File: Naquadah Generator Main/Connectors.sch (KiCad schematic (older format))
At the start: 23 parts, among them J0 Conn_ISP_Prog, J1 State_Sensing_Conn, J10 Power Board Conn, J2 State_Sensing_Conn

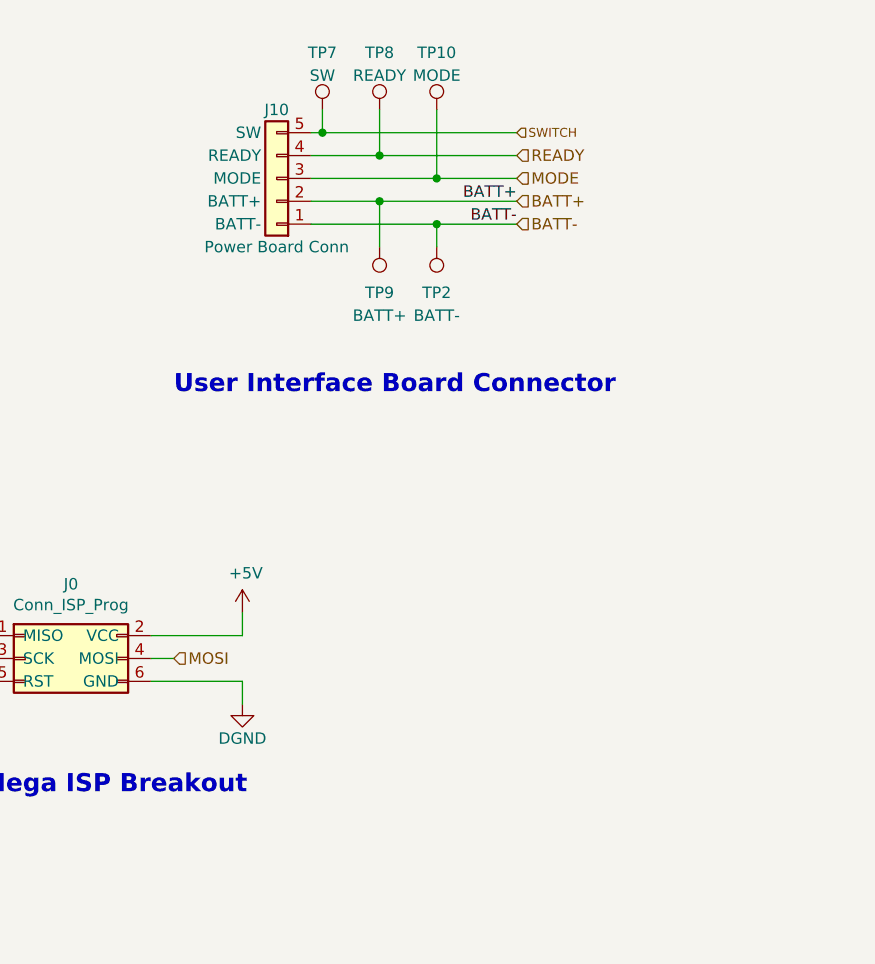
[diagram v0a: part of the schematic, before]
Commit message: Switched to 0603_1608M size for passives
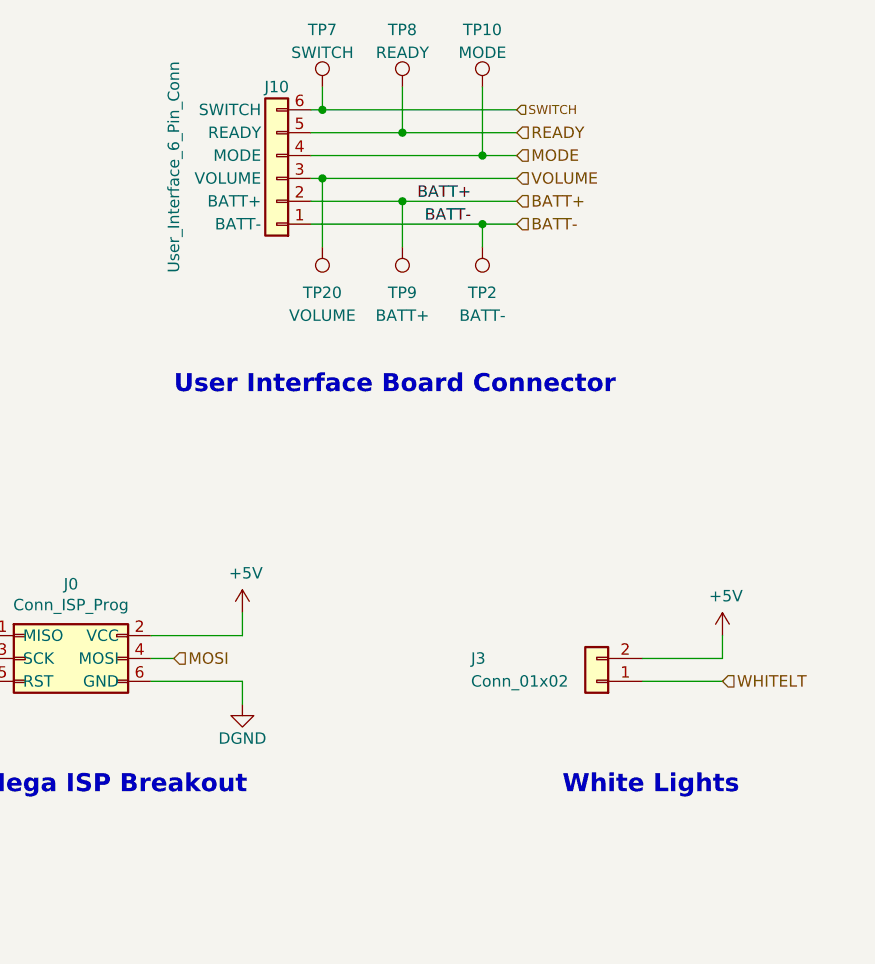
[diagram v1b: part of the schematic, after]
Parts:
- removed J10: Power Board Conn, Naquadah_Generator:Daughter_Board_Vert_5_Pin_JST_Conn, symbol Naquadah_Generator:Power_Daughter_5_Pin_Conn
- added J10: User_Interface_6_Pin_Conn, Naquadah_Generator:Daughter_Board_Vert_6_Pin_JST_Conn, symbol Naquadah_Generator:User_Interface_6_Pin_Conn
- added J3: Conn_01x02, Connector_LE:JST_SH_BM02B-SRSS-TB_1x02-1MP_P1.00mm_Vertical, symbol Connector_Generic:Conn_01x02
- added TP10: TestPoint, Frequently_Used_LE:Pad_2.5-2.5, symbol Frequently_Used_LE:TestPoint_1
- J1, J2: Description State sensing daughter board connector -> Connector Header Surface Mount, Right Angle 4 position 0.03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
- TP2, TP3, TP4, TP5, TP6, TP8, TP9: Description None -> Test point
- TP20: renamed from TP10; Description None -> Test point; Name MODE -> VOLUME
- TP7: Description None -> Test point; Name SW -> SWITCH
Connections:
- net +5V: now also J3.2 (Pin_2)
- net BATT+: now also J10.2 (BATT+)
- net BATT-: now also J10.1 (BATT-)
- net MODE: now also J10.4 (MODE), TP10.1; no longer TP20.1
- net READY: now also J10.5 (READY)
- net SWITCH: now also J10.6 (SWITCH)
- new net VOLUME: J10.3 (VOLUME), TP20.1
- new net WHITELT: J3.1 (Pin_1)
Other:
- note added: "White Lights"
- moved on the sheet: TP2, TP20, TP7, TP8, TP9

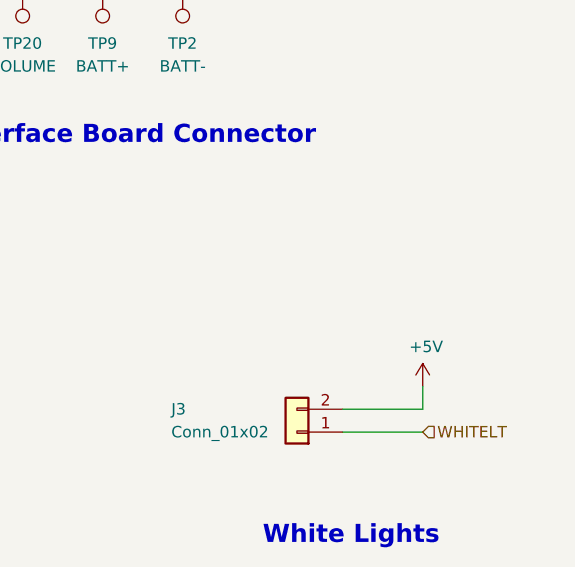
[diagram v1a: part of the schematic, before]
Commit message: Update JST connectors
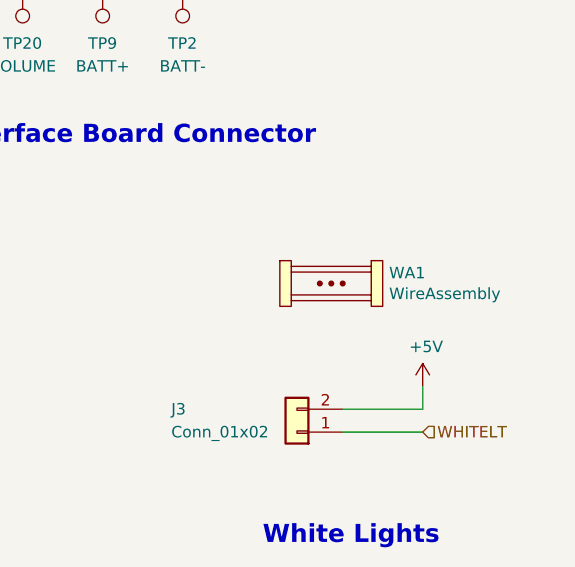
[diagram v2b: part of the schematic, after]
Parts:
- added WA1: WireAssembly, Mechanical_LE:Wire_Assembly, symbol Mechanical_LE:WireAssembly
- J1, J2: footprint Naquadah_Generator:Daughter_Board_Hor_4_Pin_JST_Conn -> Connector_JST:JST_SH_SM04B-SRSS-TB_1x04-1MP_P1.00mm_Horizontal
- J10: footprint Naquadah_Generator:Daughter_Board_Vert_6_Pin_JST_Conn -> Connector_JST:JST_SH_BM06B-SRSS-TB_1x06-1MP_P1.00mm_Vertical
